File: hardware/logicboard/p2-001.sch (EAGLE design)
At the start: 25 parts, among them IC1 5V, IC2 74LS07N, K1 G5V1, T1 2SC1815, U1 DS18B20

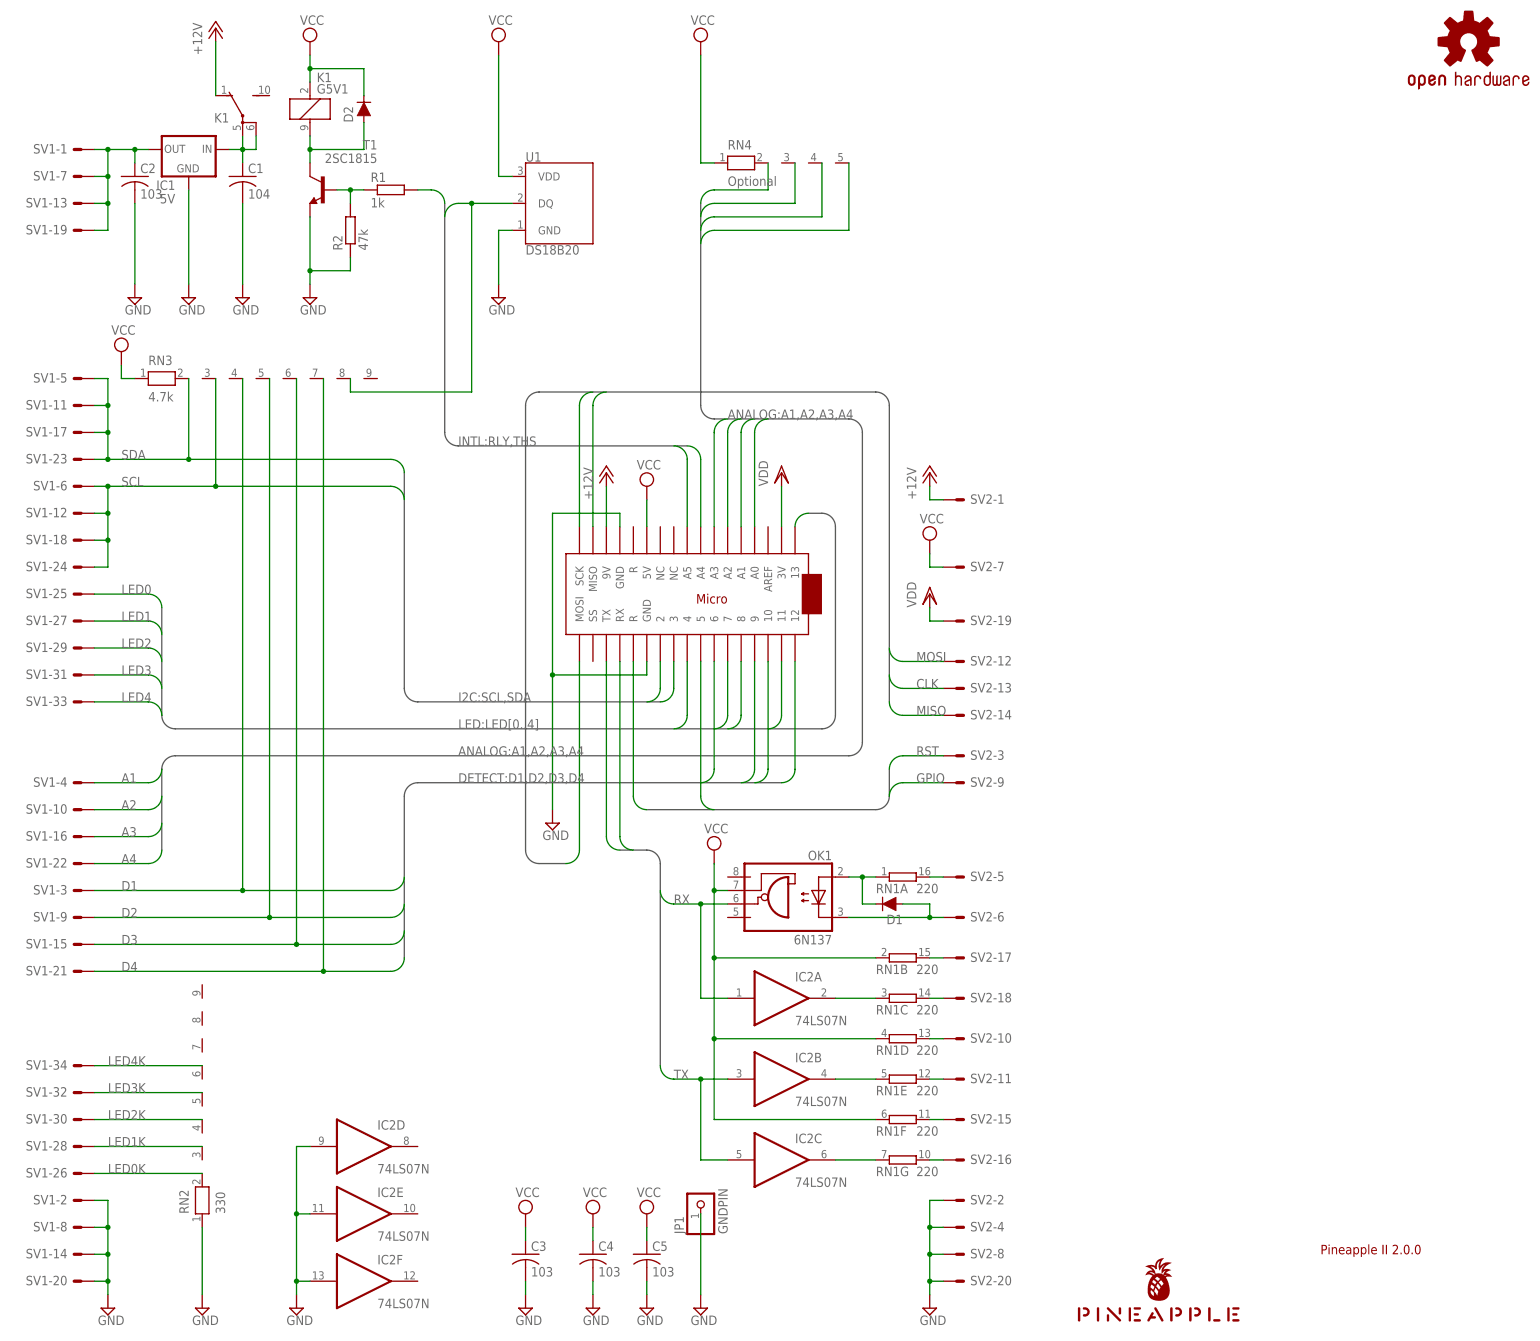
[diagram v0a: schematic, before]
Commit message: XLED terminals.
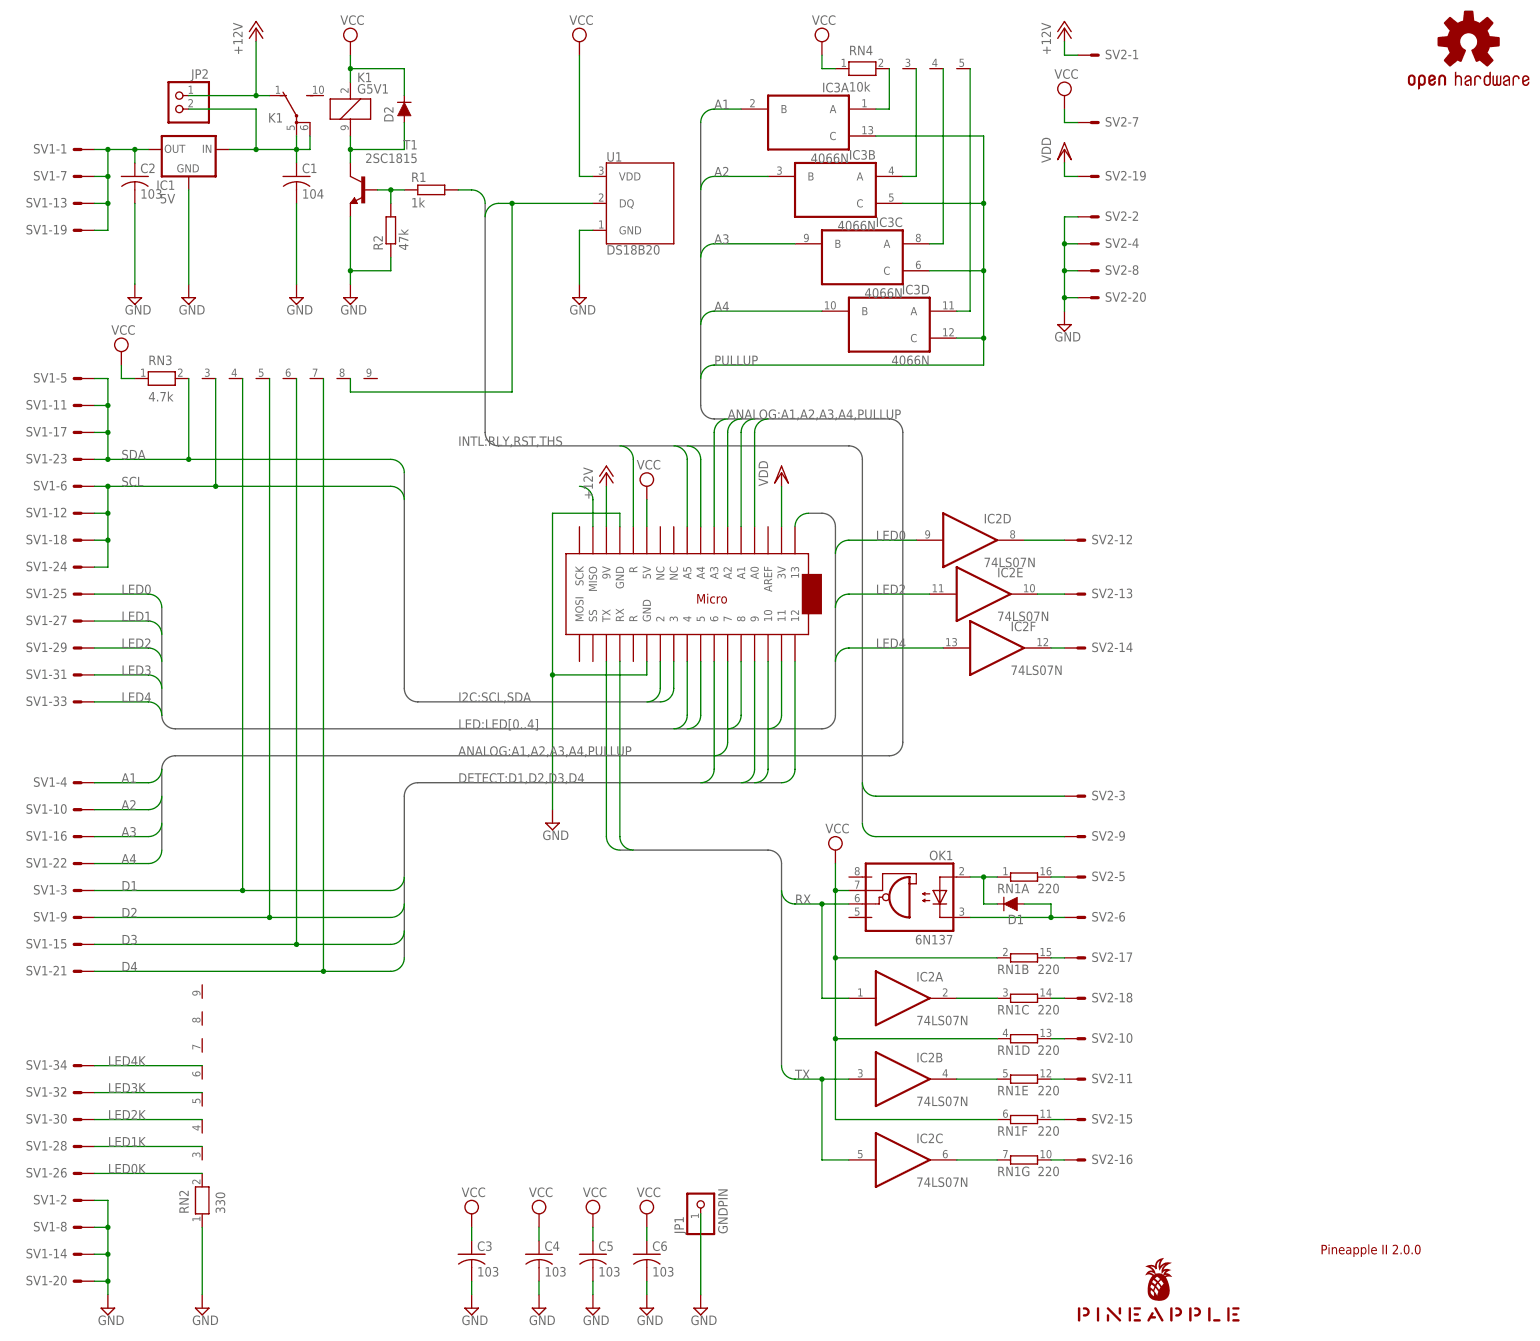
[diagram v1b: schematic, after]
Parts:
- added C6: 103, rcl:C-US025-025X050
- added IC3: 4066N, 40xx:4066N
- added JP2: (no value), pinhead:PINHD-1X2
- RN4: value Optional -> 10k
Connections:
- removed net CLK: MC1.SCK, SV2-13.S
- removed net GPIO: MC1.5, SV2-9.S
- removed net MOSI: MC1.MOSI, SV2-12.S
- new net N$13: IC2D.O, SV2-12.S
- new net N$14: IC2E.O, SV2-13.S
- new net N$15: IC2F.O, SV2-14.S
- new net N$3: IC3A.A, RN4.2
- new net N$4: IC3B.A, RN4.3
- new net N$5: IC3C.A, RN4.4
- new net N$6: IC3D.A, RN4.5
- new net PULLUP: IC3A.C, IC3B.C, IC3C.C, IC3D.C, MC1.7
- net +12V: now also JP2.1
- net 12VRLY: now also JP2.2
- net A1: now also IC3A.B; no longer RN4.2
- net A2: now also IC3B.B; no longer RN4.3
- net A3: now also IC3C.B; no longer RN4.4
- net A4: now also IC3D.B; no longer RN4.5
- net GND: now also C6.2; no longer IC2D.I, IC2E.I, IC2F.I
- net LED0: now also IC2D.I
- net LED2: now also IC2E.I, MC1.5; no longer MC1.7
- net LED4: now also IC2F.I
- net MISO: no longer SV2-14.S
- net RST: now also MC1.R@1; no longer MC1.R@2
- net THS: now also SV2-9.S
- net VCC: now also C6.1
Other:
- moved on the sheet: C1, C3, C4, C5, D1, D2, IC2A, IC2B, IC2C, IC2D, IC2E, IC2F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
